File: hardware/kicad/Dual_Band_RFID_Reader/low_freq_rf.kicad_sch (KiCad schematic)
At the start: 22 parts, among them Q1 BC517, U2 LM393, U3 LM324

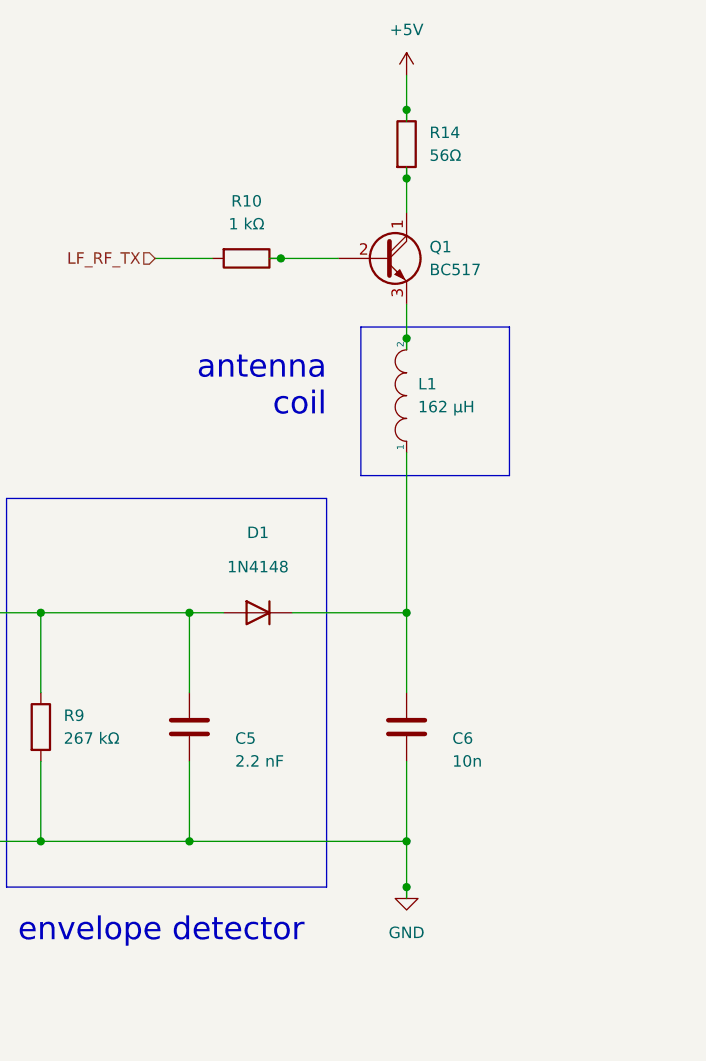
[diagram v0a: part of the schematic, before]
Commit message: Updates traces
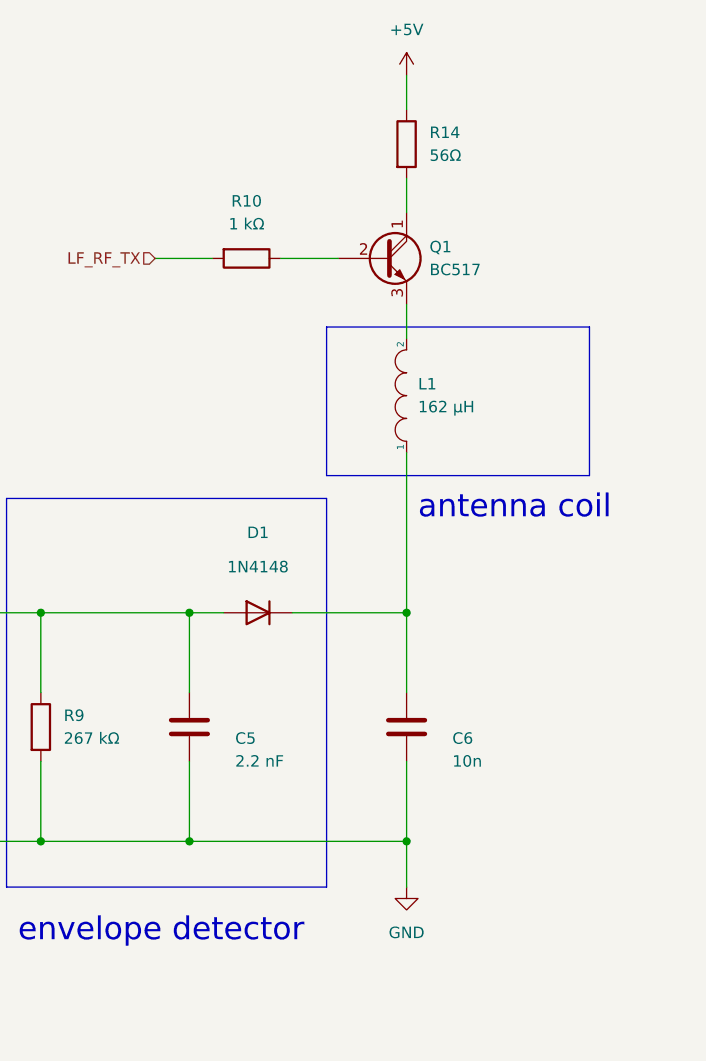
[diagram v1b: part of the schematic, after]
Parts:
- D1: footprint Diode_SMD:D_SOD-123 -> ZenerDiodes:DIOAD829W49L456D191
- L1: footprint Capstone Footprint Lib:LF Antenna Pads -> (none)
- Q1: footprint Package_TO_SOT_SMD:SOT-223 -> Package_TO_SOT_THT:TO-92_Inline; Digi-Key URL https://www.digikey.com/en/products/detail/onsemi/SPZT2222A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 -> (none); Digi-Key part number SPZT2222AT1GO -> (none); datasheet URL https://www.onsemi.com/pdf/datasheet/pzt2222at1-d.pdf -> (none)
- U2: footprint Package_SO:SOIC-8_3.9x4.9mm_P1.27mm -> DualComparator_LM393:SO08; Digi-Key URL https://www.digikey.com/en/products/detail/onsemi/LM393EDR2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 -> (none); Digi-Key part number LM393EDR2GO -> (none); datasheet URL https://www.onsemi.com/pdf/datasheet/lm393-d.pdf -> (none)
- U3: footprint Package_SO:SOIC-14_3.9x8.7mm_P1.27mm -> GPOPAmp_LM324:SOIC127P600X175-14N; Digi-Key URL https://www.digikey.com/en/products/detail/onsemi/LM324DR2G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 -> (none); Digi-Key part number LM324DR2GO -> (none)
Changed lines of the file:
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@@
   (junction (at 41.91 101.6) (diameter 0) (color 0 0 0 0)
   )
-  (junction (at 233.68 57.15) (diameter 0) (color 0 0 0 0)
-  )
   (junction (at 247.65 96.52) (diameter 0) (color 0 0 0 0)
   )
@@
   (junction (at 76.2 130.81) (diameter 0) (color 0 0 0 0)
   )
-  (junction (at 247.65 66.04) (diameter 0) (color 0 0 0 0)
-  )
   (junction (at 223.52 96.52) (diameter 0) (color 0 0 0 0)
   )
@@
   (junction (at 119.38 111.76) (diameter 0) (color 0 0 0 0)
   )
-  (junction (at 247.65 40.64) (diameter 0) (color 0 0 0 0)
-  )
   (junction (at 207.01 96.52) (diameter 0) (color 0 0 0 0)
   )
-  (junction (at 247.65 127) (diameter 0) (color 0 0 0 0)
-  )
-  (junction (at 247.65 48.26) (diameter 0) (color 0 0 0 0)
-  )
   (junction (at 247.65 121.92) (diameter 0) (color 0 0 0 0)
   )
@@
     (stroke (width 0) (type default))
   )
-  (wire (pts (xy 232.41 57.15) (xy 233.68 57.15))
-    (stroke (width 0) (type default))
-  )
   (wire (pts (xy 219.71 57.15) (xy 226.06 57.15))
     (stroke (width 0) (type default))
@@
     (stroke (width 0) (type default))
   )
-  (wire (pts (xy 247.65 46.99) (xy 247.65 48.26))
-    (stroke (width 0) (type default))
-  )
   (wire (pts (xy 207.01 96.52) (xy 207.01 105.41))
     (stroke (width 0) (type default))
@@
     (stroke (width 0) (type default))
   )
-  (wire (pts (xy 247.65 40.64) (xy 247.65 41.91))
-    (stroke (width 0) (type default))
-  )
   (wire (pts (xy 207.01 113.03) (xy 207.01 121.92))
     (stroke (width 0) (type default))
@@
     (stroke (width 0) (type default))
   )
-  (polyline (pts (xy 242.57 64.77) (xy 242.57 81.28))
-    (stroke (width 0) (type default))
-  )
-  (polyline (pts (xy 242.57 64.77) (xy 259.08 64.77))
-    (stroke (width 0) (type default))
-  )
-  (polyline (pts (xy 259.08 64.77) (xy 259.08 81.28))
-    (stroke (width 0) (type default))
-  )
-  (polyline (pts (xy 259.08 81.28) (xy 242.57 81.28))
+  (polyline (pts (xy 238.76 64.77) (xy 238.76 81.28))
+    (stroke (width 0) (type default))
+  )
+  (polyline (pts (xy 238.76 64.77) (xy 267.97 64.77))
+    (stroke (width 0) (type default))
+  )
+  (polyline (pts (xy 267.97 64.77) (xy 267.97 81.28))
+    (stroke (width 0) (type default))
+  )
+  (polyline (pts (xy 267.97 81.28) (xy 238.76 81.28))
     (stroke (width 0) (type default))
   )
@@
     (stroke (width 0) (type default))
   )
-  (wire (pts (xy 247.65 127) (xy 247.65 128.27))
-    (stroke (width 0) (type default))
-  )
   (wire (pts (xy 233.68 57.15) (xy 240.03 57.15))
     (stroke (width 0) (type default))
@@
   )
   (wire (pts (xy 41.91 97.79) (xy 41.91 101.6))
-    (stroke (width 0) (type default))
-  )
-  (wire (pts (xy 247.65 66.04) (xy 247.65 67.31))
     (stroke (width 0) (type default))
   )
@@
     (effects (font (size 2.54 2.54)) (justify left bottom))
   )
-  (text "antenna\ncoil" (at 238.76 74.93 0)
-    (effects (font (size 2.54 2.54)) (justify right bottom))
+  (text "antenna coil" (at 248.92 86.36 0)
+    (effects (font (size 2.54 2.54)) (justify left bottom))
   )
   (text "envelope detector" (at 204.47 133.35 0)
@@
       (effects (font (size 1.27 1.27)))
     )
-    (property "Footprint" "Package_SO:SOIC-8_3.9x4.9mm_P1.27mm" (id 2) (at 60.96 101.6 0)
-      (effects (font (size 1.27 1.27)) hide)
-    )
-    (property "Datasheet" "https://www.onsemi.com/pdf/datasheet/lm393-d.pdf" (id 3) (at 60.96 101.6 0)
-      (effects (font (size 1.27 1.27)) hide)
-    )
-    (property "Digi-Key part number" "LM393EDR2GO" (id 4) (at 60.96 101.6 0)
-      (effects (font (size 1.27 1.27)) hide)
-    )
-    (property "Digi-Key URL" "https://www.digikey.com/en/products/detail/onsemi/LM393EDR2G/7220419" (id 5) (at 60.96 101.6 0)
-      (effects (font (size 1.27 1.27)) hide)
-    )
-    (property "datasheet URL" "https://www.onsemi.com/pdf/datasheet/lm393-d.pdf" (id 6) (at 60.96 101.6 0)
+    (property "Footprint" "DualComparator_LM393:SO08" (id 2) (at 60.96 101.6 0)
+      (effects (font (size 1.27 1.27)) hide)
+    )
+    (property "Datasheet" "http://www.ti.com/lit/ds/symlink/lm393.pdf" (id 3) (at 60.96 101.6 0)
       (effects (font (size 1.27 1.27)) hide)
     )
@@
     (pin "2")
     (pin "3")
+    (pin "5")
+    (pin "6")
+    (pin "7")
+    (pin "4")
+    (pin "8")
   )
   (symbol (lib_id "Device:D") (at 231.14 96.52 0) (mirror y) (unit 1)
@@
       (effects (font (size 1.27 1.27)))
     )
-    (property "Footprint" "Diode_SMD:D_SOD-123" (id 2) (at 231.14 96.52 0)
+    (property "Footprint" "ZenerDiodes:DIOAD829W49L456D191" (id 2) (at 231.14 96.52 0)
       (effects (font (size 1.27 1.27)) hide)
     )
@@
       (effects (font (size 1.27 1.27)) (justify right))
     )
-    (property "Footprint" "Capstone Footprint Lib:LF Antenna Pads" (id 2) (at 247.65 72.39 0)
+    (property "Footprint" "" (id 2) (at 247.65 72.39 0)
       (effects (font (size 1.27 1.27)) hide)
     )
@@
       (effects (font (size 1.27 1.27)))
     )
-    (property "Footprint" "Package_SO:SOIC-14_3.9x8.7mm_P1.27mm" (id 2) (at 109.22 96.52 0)
-      (effects (font (size 1.27 1.27)) hide)
-    )
-    (property "Datasheet" "https://www.onsemi.com/pdf/datasheet/lm324-d.pdf" (id 3) (at 106.68 93.98 0)
-      (effects (font (size 1.27 1.27)) hide)
-    )
-    (property "Digi-Key part number" "LM324DR2GO" (id 4) (at 107.95 99.06 0)
-      (effects (font (size 1.27 1.27)) hide)
-    )
-    (property "Digi-Key URL" "https://www.digikey.com/en/products/detail/onsemi/LM324DR2G/918511" (id 5) (at 107.95 99.06 0)
+    (property "Footprint" "GPOPAmp_LM324:SOIC127P600X175-14N" (id 2) (at 109.22 96.52 0)
+      (effects (font (size 1.27 1.27)) hide)
+    )
+    (property "Datasheet" "http://www.ti.com/lit/ds/symlink/lm2902-n.pdf" (id 3) (at 106.68 93.98 0)
       (effects (font (size 1.27 1.27)) hide)
     )
@@
     (pin "2")
     (pin "3")
+    (pin "5")
+    (pin "6")
+    (pin "7")
+    (pin "10")
+    (pin "8")
+    (pin "9")
+    (pin "12")
+    (pin "13")
+    (pin "14")
+    (pin "11")
+    (pin "4")
   )
   (symbol (lib_id "power:+3.3V") (at 76.2 115.57 0) (unit 1)
@@
       (effects (font (size 1.27 1.27)) (justify left))
     )
-    (property "Footprint" "Package_TO_SOT_SMD:SOT-223" (id 2) (at 250.19 59.055 0)
+    (property "Footprint" "Package_TO_SOT_THT:TO-92_Inline" (id 2) (at 250.19 59.055 0)
       (effects (font (size 1.27 1.27) italic) (justify left) hide)
     )
-    (property "Datasheet" "" (id 3) (at 245.11 57.15 0)
+    (property "Datasheet" "https://www.onsemi.com/pub/Collateral/BC517-D74Z-D.PDF" (id 3) (at 245.11 57.15 0)
       (effects (font (size 1.27 1.27)) (justify left) hide)
     )
-    (property "Digi-Key part number" "SPZT2222AT1GO" (id 4) (at 245.11 57.15 0)
-      (effects (font (size 1.27 1.27)) hide)
-    )
-    (property "Digi-Key URL" "https://www.digikey.com/en/products/detail/onsemi/SPZT2222AT1G/3062863" (id 5) (at 245.11 57.15 0)
-      (effects (font (size 1.27 1.27)) hide)
-    )
-    (property "datasheet URL" "https://www.onsemi.com/pdf/datasheet/pzt2222at1-d.pdf" (id 6) (at 245.11 57.15 0)
-      (effects (font (size 1.27 1.27)) hide)
-    )
-    (pin "1")
+    (pin "1")
